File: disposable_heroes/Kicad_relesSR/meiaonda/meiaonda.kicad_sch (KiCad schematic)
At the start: 44 parts, among them J1 Canal 1 - V_{in}, J10 Gerador Sinal, J2 Fonte 12V, J3 Fonte 5V - VB, J4 GPIO22, J5 GPIO26, J6 GPIO6, J7 GPIO13, J8 GPIO27, J9 Canal 2 - V_{out}, K1 3572-1220-123, K10 3572-1220-123, K11 3572-1220-123, K12 3570-1331-123, K13 3570-1331-123, K14 3570-1331-123, K2 3572-1220-123, K3 3572-1220-123, K4 3570-1331-123, K5 3572-1220-123, K6 3572-1220-123, K7 3572-1220-123, K8 3572-1220-123, K9 3572-1220-123, U1 74HC595N_112, U2 ULN2003, U3 74HC595N_112, U4 ULN2003

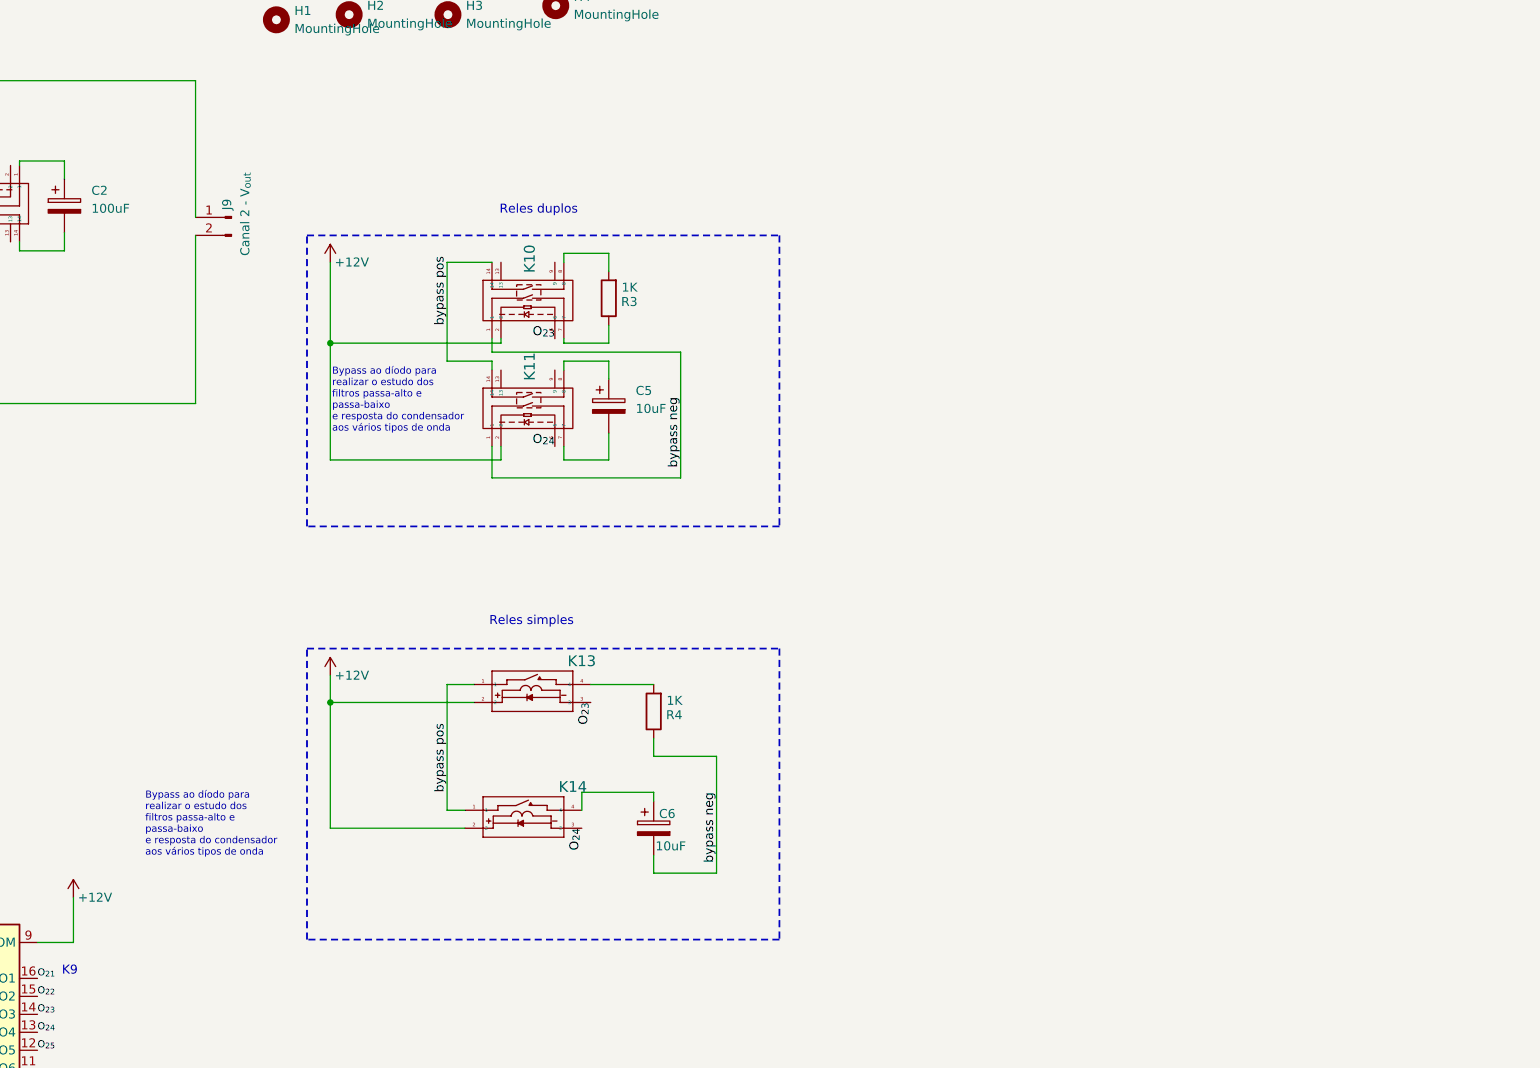
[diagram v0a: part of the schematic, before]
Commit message: problemas com o onda completa
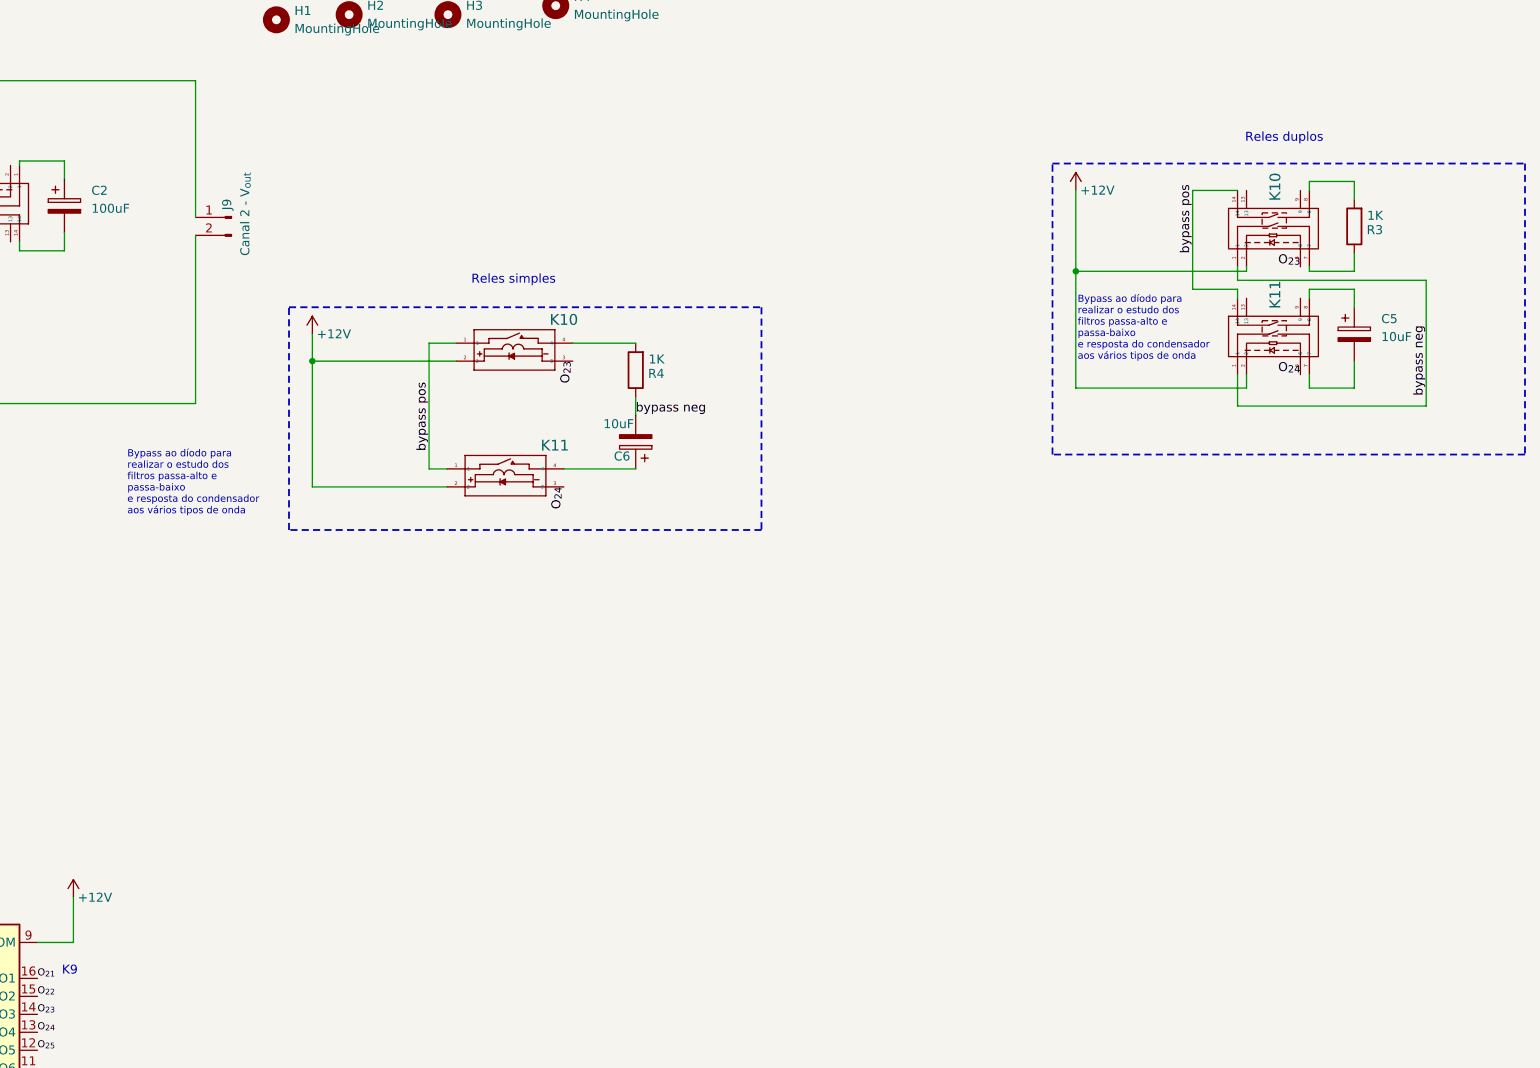
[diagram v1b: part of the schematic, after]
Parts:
- renumbered K13 to K10, K14 to K11
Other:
- moved on the sheet: C5, C6, K10, K11, R3, R4
